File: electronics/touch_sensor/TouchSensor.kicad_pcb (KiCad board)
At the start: 2 copper layers, 26.5 x 19.2 mm, 8 parts, among them J1 Conn_01x03_Pin, Q1 BSS127S, Q2 BSS127S

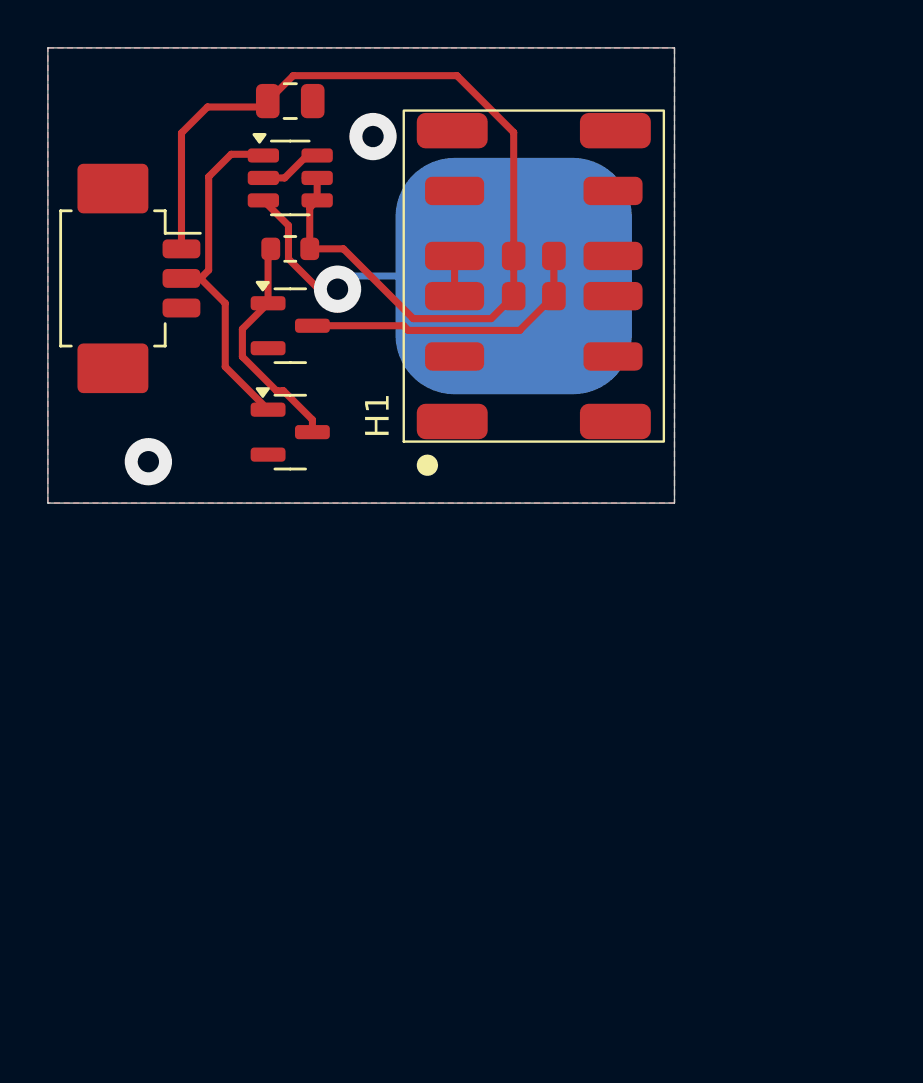
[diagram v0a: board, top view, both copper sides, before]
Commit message: updated pcb
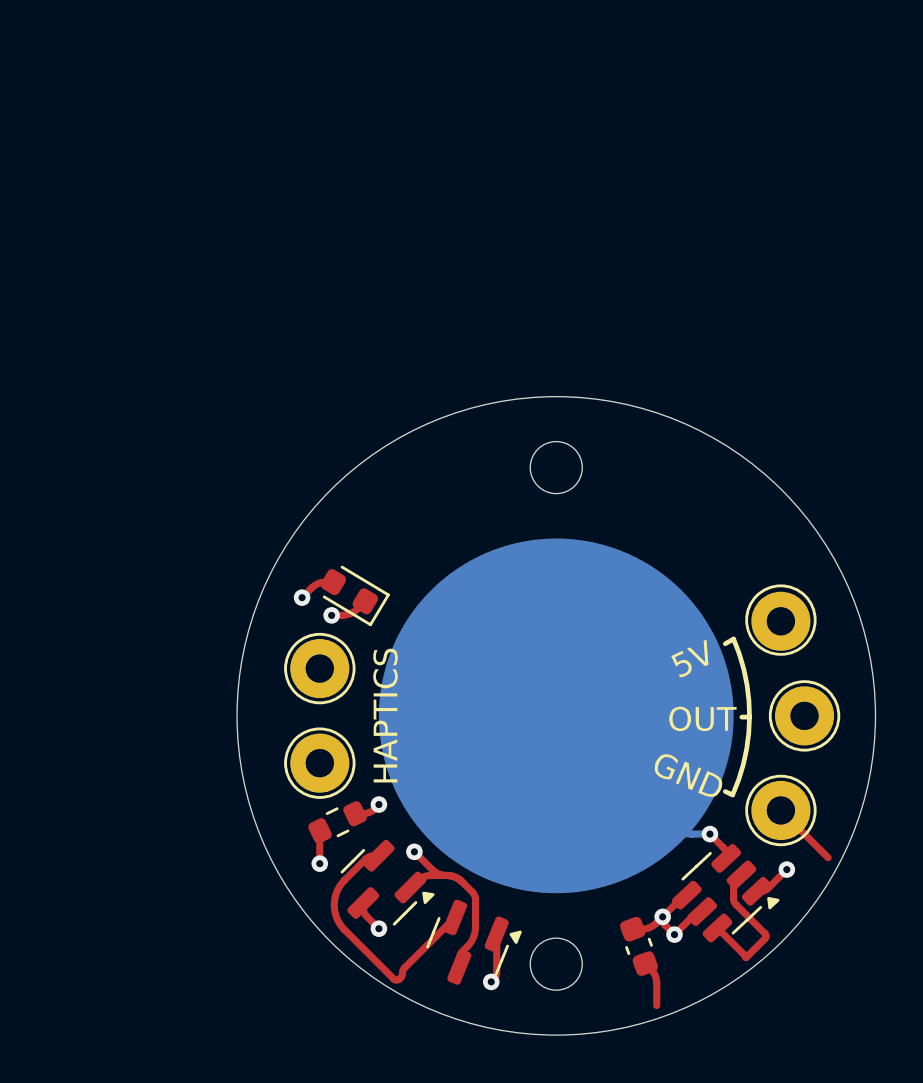
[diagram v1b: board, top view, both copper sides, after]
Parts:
- removed J1: Conn_01x03_Pin, Connector_Molex:Molex_PicoBlade_53261-0371_1x03-1MP_P1.25mm_Horizontal
- added D1: LED, Diode_SMD:D_0603_1608Metric, F.Cu at (146.2, 102.0)
- added H2: MountingHole, MountingHole:MountingHole_2.2mm_M2_ISO7380, F.Cu at (155.0, 117.8)
- added TP1: TestPoint, TestPoint:TestPoint_THTPad_D2.5mm_Drill1.2mm, F.Cu at (164.5, 103.2)
- added TP2: TestPoint, TestPoint:TestPoint_THTPad_D2.5mm_Drill1.2mm, F.Cu at (165.5, 107.2)
- added TP3: TestPoint, TestPoint:TestPoint_THTPad_D2.5mm_Drill1.2mm, F.Cu at (164.5, 111.2)
- added TP4: TestPoint, TestPoint:TestPoint_THTPad_D2.5mm_Drill1.2mm, F.Cu at (145.0, 105.2)
- added TP5: TestPoint, TestPoint:TestPoint_THTPad_D2.5mm_Drill1.2mm, F.Cu at (145.0, 109.2)
- C2: footprint Capacitor_SMD:C_0805_2012Metric -> Capacitor_SMD:C_0603_1608Metric
- H1: value ~ -> MountingHole; footprint TouchSensor:ELV1411A -> MountingHole:MountingHole_2.2mm_M2_ISO7380
- moved C2 38.7 mm to (158.5, 117.0), turned to -70 degrees
- moved U1 35.3 mm to (162.0, 114.8), turned to -137 degrees
- moved R1 24.3 mm to (145.8, 111.8), turned to -154 degrees
- moved Q1 24.0 mm to (147.5, 114.5), turned to -135 degrees
- moved Q2 23.0 mm to (151.2, 117.0), turned to -112 degrees
- moved T1 18.7 mm to (155.0, 107.2), turned to 180 degrees
- moved H1 8.16 mm to (155.0, 96.8), turned to 0 degrees
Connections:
- Q1 pad 3: Net-(Q1-D) -> Net-(D1-K)
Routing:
- net +5V: track 41.8 -> 19.8 mm, vias 0 -> 3
- net GND: track 4.37 -> 21.9 mm, vias 2 -> 0
- net Net-(D1-K): track 0.00 -> 16.9 mm, vias 0 -> 2
- net Net-(Q1-D): track 12.6 -> 0.00 mm
- net /Output: track 14.7 -> 26.4 mm, vias 0 -> 2
- net Net-(D1-A): track 0.00 -> 9.64 mm, vias 0 -> 1
- net Net-(Q1-G): track 9.65 -> 14.4 mm, vias 0 -> 2
- net /Sens: track 13.2 -> 9.78 mm
- removed copper zone on B.Cu, net GND
- removed copper zone on F.Cu, net GND
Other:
- board size 26.5 x 19.2 mm -> 27 x 27 mm
- copper layers 2 -> 4
- board text added: "5V"
- board text added: "GND"
- board text added: "HAPTICS"
- board text added: "OUT"
